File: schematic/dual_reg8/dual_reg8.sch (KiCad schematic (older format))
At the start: 52 parts

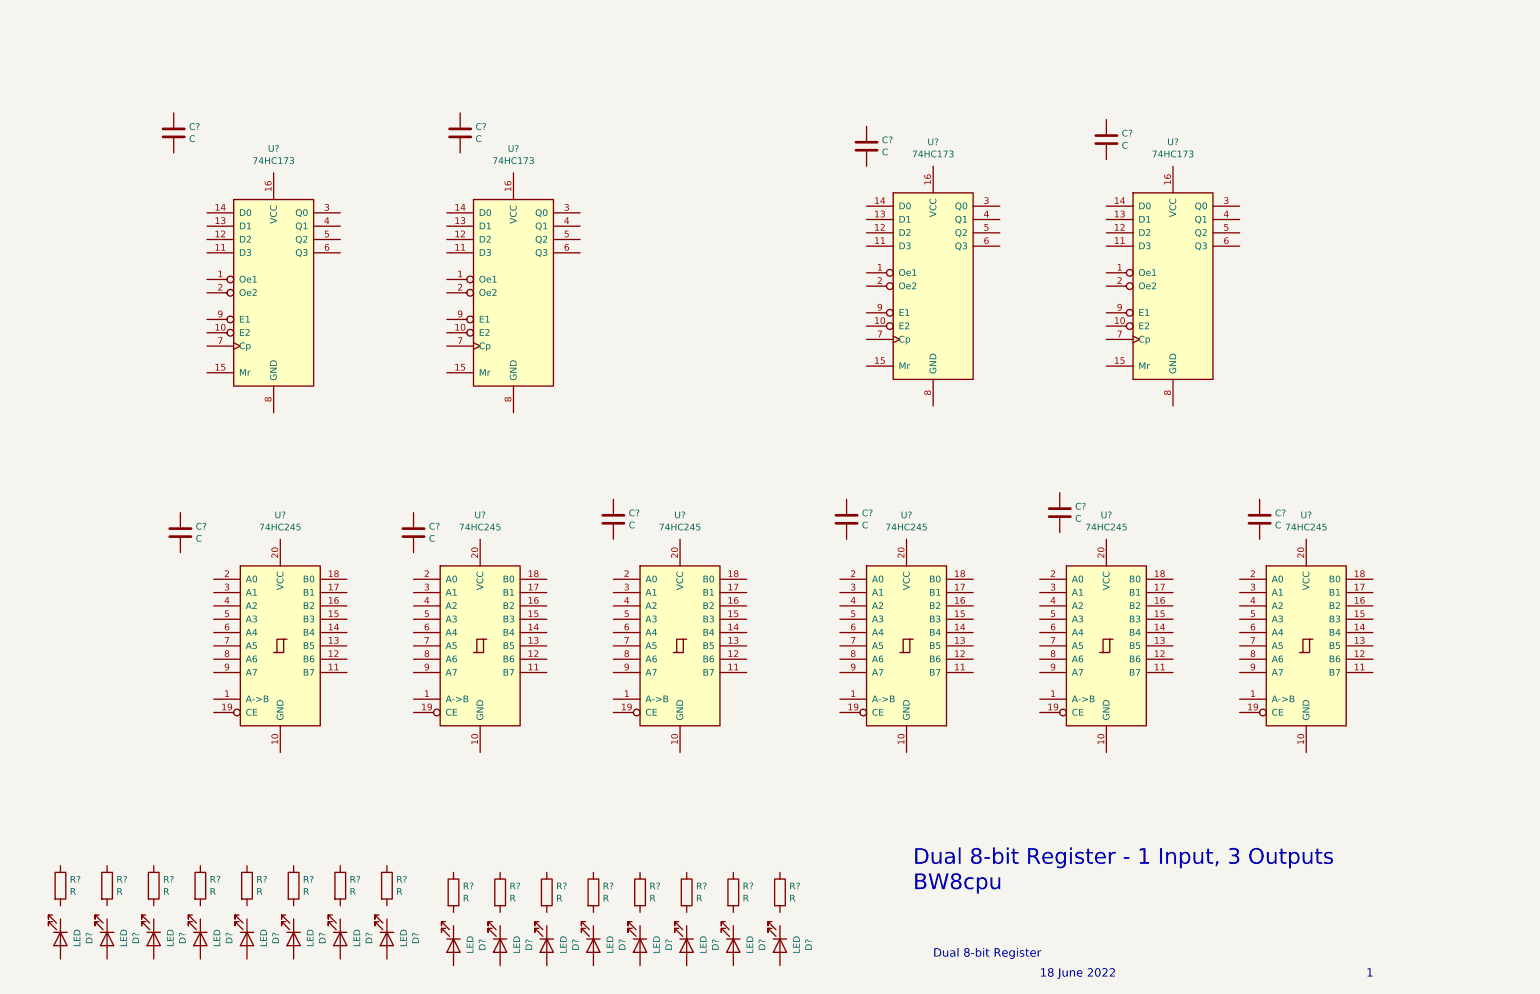
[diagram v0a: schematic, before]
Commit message: switching branches, cleaning tree
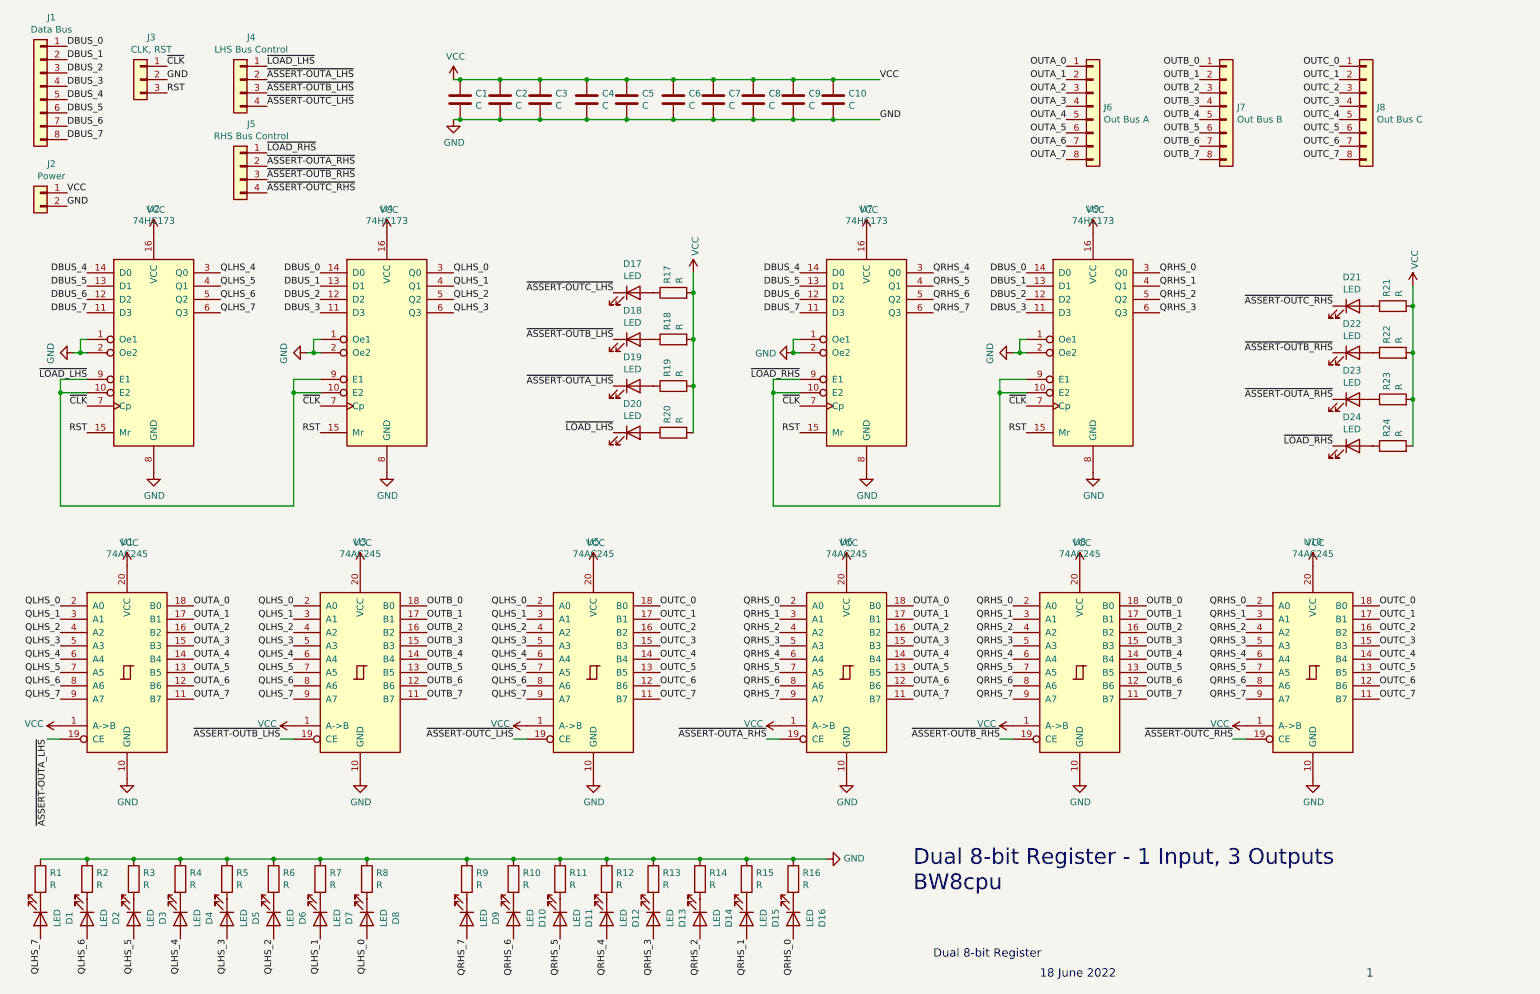
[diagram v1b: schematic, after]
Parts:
- removed C? (x9): C, symbol Device:C
- removed D? (x15): LED, symbol Device:LED
- removed R? (x15): R, symbol Device:R
- removed U? (x2): 74HC173, symbol 74xx:74LS173
- removed U? (x3): 74HC245, symbol 74xx:74HC245
- added C10, C2, C3, C4, C5, C6, C7, C8, C9: C, Capacitor_THT:C_Disc_D3.0mm_W1.6mm_P2.50mm, symbol Device:C
- added D10, D11, D12, D13, D14, D15, D16, D17, D18, D19, D2, D20, D21, D22, D23, D24, D3, D4, D5, D6, D7, D8, D9: LED, LED_THT:LED_D2.0mm_W4.8mm_H2.5mm_FlatTop, symbol Device:LED
- added J1: Data Bus, Connector_PinSocket_2.54mm:PinSocket_1x08_P2.54mm_Vertical, symbol Connector_Generic:Conn_01x08
- added J2: Power, Connector_PinSocket_2.54mm:PinSocket_1x02_P2.54mm_Vertical, symbol Connector_Generic:Conn_01x02
- added J3: CLK, RST, Connector_PinSocket_2.54mm:PinSocket_1x03_P2.54mm_Vertical, symbol Connector_Generic:Conn_01x03
- added J4: LHS Bus Control, Connector_PinSocket_2.54mm:PinSocket_1x04_P2.54mm_Vertical, symbol Connector_Generic:Conn_01x04
- added J5: RHS Bus Control, Connector_PinSocket_2.54mm:PinSocket_1x04_P2.54mm_Vertical, symbol Connector_Generic:Conn_01x04
- added J6: Out Bus A, Connector_PinSocket_2.54mm:PinSocket_1x08_P2.54mm_Vertical, symbol Connector_Generic:Conn_01x08
- added J7: Out Bus B, Connector_PinSocket_2.54mm:PinSocket_1x08_P2.54mm_Vertical, symbol Connector_Generic:Conn_01x08
- added J8: Out Bus C, Connector_PinSocket_2.54mm:PinSocket_1x08_P2.54mm_Vertical, symbol Connector_Generic:Conn_01x08
- added R10, R11, R12, R13, R14, R15, R16, R17, R18, R19, R2, R20, R21, R22, R23, R24, R3, R4, R5, R6, R7, R8, R9: R, Resistor_THT:R_Axial_DIN0204_L3.6mm_D1.6mm_P5.08mm_Horizontal, symbol Device:R
- added U10, U6, U8: 74AC245, Package_DIP:DIP-20_W7.62mm, symbol 74xx:74HC245
- added U7, U9: 74HC173, Package_DIP:DIP-16_W7.62mm, symbol 74xx:74LS173
- C1: renamed from C?; footprint (none) -> Capacitor_THT:C_Disc_D3.0mm_W1.6mm_P2.50mm
- D1: renamed from D?; footprint (none) -> LED_THT:LED_D2.0mm_W4.8mm_H2.5mm_FlatTop
- R1: renamed from R?; footprint (none) -> Resistor_THT:R_Axial_DIN0204_L3.6mm_D1.6mm_P5.08mm_Horizontal
- U1, U3, U5: renamed from U?; value 74HC245 -> 74AC245; footprint (none) -> Package_DIP:DIP-20_W7.62mm
- U2, U4: renamed from U?; footprint (none) -> Package_DIP:DIP-16_W7.62mm
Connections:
- net GND: now reaches U2.1 (Oe1)
- net GND: now also C1.2, R1.1, U1.10 (GND), U2.2 (Oe2), U2.8 (GND), U3.10 (GND), U4.1 (Oe1), U4.2 (Oe2), U4.8 (GND), U5.10 (GND), C10.2, C2.2, C3.2, C4.2, C5.2, C6.2, C7.2, C8.2, C9.2, J2.2 (Pin_2), J3.2 (Pin_2), R10.1, R11.1, R12.1, R13.1, R14.1, R15.1, R16.1, R2.1, R3.1, R4.1, R5.1, R6.1, R7.1, R8.1, R9.1, U10.10 (GND), U6.10 (GND), U7.1 (Oe1), U7.2 (Oe2), U7.8 (GND), U8.10 (GND), U9.1 (Oe1), U9.2 (Oe2), U9.8 (GND)
- net ~LOAD_LHS: now reaches U2.10 (E2)
- net ~LOAD_LHS: now also U2.9 (E1), U4.10 (E2), U4.9 (E1), D20.1 (K), J4.1 (Pin_1)
- net DBUS_7: now reaches U2.11 (D3)
- net DBUS_7: now also J1.8 (Pin_8), U7.11 (D3)
- net DBUS_6: now reaches U2.12 (D2)
- net DBUS_6: now also J1.7 (Pin_7), U7.12 (D2)
- net DBUS_5: now reaches U2.13 (D1)
- net DBUS_5: now also J1.6 (Pin_6), U7.13 (D1)
- net DBUS_4: now reaches U2.14 (D0)
- net DBUS_4: now also J1.5 (Pin_5), U7.14 (D0)
- net RST: now reaches U2.15 (Mr)
- net RST: now also U4.15 (Mr), J3.3 (Pin_3), U7.15 (Mr), U9.15 (Mr)
- net VCC: now reaches U2.16 (VCC)
- net VCC: now also C1.1, U1.1 (A->B), U1.20 (VCC), U3.1 (A->B), U3.20 (VCC), U4.16 (VCC), U5.1 (A->B), U5.20 (VCC), C10.1, C2.1, C3.1, C4.1, C5.1, C6.1, C7.1, C8.1, C9.1, J2.1 (Pin_1), R17.2, R18.2, R19.2, R20.2, R21.2, R22.2, R23.2, R24.2, U10.1 (A->B), U10.20 (VCC), U6.1 (A->B), U6.20 (VCC), U7.16 (VCC), U8.1 (A->B), U8.20 (VCC), U9.16 (VCC)
- net QLHS_4: now reaches U2.3 (Q0)
- net QLHS_4: now also U1.6 (A4), U3.6 (A4), U5.6 (A4), D4.2 (A)
- net QLHS_5: now reaches U2.4 (Q1)
- net QLHS_5: now also U1.7 (A5), U3.7 (A5), U5.7 (A5), D3.2 (A)
- net QLHS_6: now reaches U2.5 (Q2)
- net QLHS_6: now also U1.8 (A6), U3.8 (A6), U5.8 (A6), D2.2 (A)
- net QLHS_7: now reaches U2.6 (Q3)
- net QLHS_7: now also D1.2 (A), U1.9 (A7), U3.9 (A7), U5.9 (A7)
- net ~CLK: now reaches U2.7 (Cp)
- net ~CLK: now also U4.7 (Cp), J3.1 (Pin_1), U7.7 (Cp), U9.7 (Cp)
- net DBUS_3: now reaches U4.11 (D3)
- net DBUS_3: now also J1.4 (Pin_4), U9.11 (D3)
- net DBUS_2: now reaches U4.12 (D2)
- net DBUS_2: now also J1.3 (Pin_3), U9.12 (D2)
- net DBUS_1: now reaches U4.13 (D1)
- net DBUS_1: now also J1.2 (Pin_2), U9.13 (D1)
- net DBUS_0: now reaches U4.14 (D0)
- net DBUS_0: now also J1.1 (Pin_1), U9.14 (D0)
- net QLHS_0: now reaches U4.3 (Q0)
- net QLHS_0: now also U1.2 (A0), U3.2 (A0), U5.2 (A0), D8.2 (A)
- net QLHS_1: now reaches U4.4 (Q1)
- net QLHS_1: now also U1.3 (A1), U3.3 (A1), U5.3 (A1), D7.2 (A)
- net QLHS_2: now reaches U4.5 (Q2)
- net QLHS_2: now also U1.4 (A2), U3.4 (A2), U5.4 (A2), D6.2 (A)
- net QLHS_3: now reaches U4.6 (Q3)
- net QLHS_3: now also U1.5 (A3), U3.5 (A3), U5.5 (A3), D5.2 (A)
- net OUTA_7: now reaches U1.11 (B7)
- net OUTA_7: now also J6.8 (Pin_8), U6.11 (B7)
- net OUTA_6: now reaches U1.12 (B6)
- net OUTA_6: now also J6.7 (Pin_7), U6.12 (B6)
- net OUTA_5: now reaches U1.13 (B5)
- net OUTA_5: now also J6.6 (Pin_6), U6.13 (B5)
- net OUTA_4: now reaches U1.14 (B4)
- net OUTA_4: now also J6.5 (Pin_5), U6.14 (B4)
- net OUTA_3: now reaches U1.15 (B3)
- net OUTA_3: now also J6.4 (Pin_4), U6.15 (B3)
- net OUTA_2: now reaches U1.16 (B2)
- net OUTA_2: now also J6.3 (Pin_3), U6.16 (B2)
- net OUTA_1: now reaches U1.17 (B1)
- net OUTA_1: now also J6.2 (Pin_2), U6.17 (B1)
- net OUTA_0: now reaches U1.18 (B0)
- net OUTA_0: now also J6.1 (Pin_1), U6.18 (B0)
- net ~ASSERT-OUTA_LHS: now reaches U1.19 (CE)
- net ~ASSERT-OUTA_LHS: now also D19.1 (K), J4.2 (Pin_2)
- net OUTB_7: now reaches U3.11 (B7)
- net OUTB_7: now also J7.8 (Pin_8), U8.11 (B7)
- net OUTB_6: now reaches U3.12 (B6)
- net OUTB_6: now also J7.7 (Pin_7), U8.12 (B6)
- net OUTB_5: now reaches U3.13 (B5)
- net OUTB_5: now also J7.6 (Pin_6), U8.13 (B5)
- net OUTB_4: now reaches U3.14 (B4)
- net OUTB_4: now also J7.5 (Pin_5), U8.14 (B4)
- net OUTB_3: now reaches U3.15 (B3)
- net OUTB_3: now also J7.4 (Pin_4), U8.15 (B3)
- net OUTB_2: now reaches U3.16 (B2)
- net OUTB_2: now also J7.3 (Pin_3), U8.16 (B2)
- net OUTB_1: now reaches U3.17 (B1)
- net OUTB_1: now also J7.2 (Pin_2), U8.17 (B1)
- net OUTB_0: now reaches U3.18 (B0)
- net OUTB_0: now also J7.1 (Pin_1), U8.18 (B0)
- net ~ASSERT-OUTB_LHS: now reaches U3.19 (CE)
- net ~ASSERT-OUTB_LHS: now also D18.1 (K), J4.3 (Pin_3)
- net OUTC_7: now reaches U5.11 (B7)
- net OUTC_7: now also J8.8 (Pin_8), U10.11 (B7)
- net OUTC_6: now reaches U5.12 (B6)
- net OUTC_6: now also J8.7 (Pin_7), U10.12 (B6)
- net OUTC_5: now reaches U5.13 (B5)
- net OUTC_5: now also J8.6 (Pin_6), U10.13 (B5)
- net OUTC_4: now reaches U5.14 (B4)
- net OUTC_4: now also J8.5 (Pin_5), U10.14 (B4)
- net OUTC_3: now reaches U5.15 (B3)
- net OUTC_3: now also J8.4 (Pin_4), U10.15 (B3)
- net OUTC_2: now reaches U5.16 (B2)
- net OUTC_2: now also J8.3 (Pin_3), U10.16 (B2)
- net OUTC_1: now reaches U5.17 (B1)
- net OUTC_1: now also J8.2 (Pin_2), U10.17 (B1)
- net OUTC_0: now reaches U5.18 (B0)
- net OUTC_0: now also J8.1 (Pin_1), U10.18 (B0)
- net ~ASSERT-OUTC_LHS: now reaches U5.19 (CE)
- net ~ASSERT-OUTC_LHS: now also D17.1 (K), J4.4 (Pin_4)
- net at D1.1 (K): now also R1.2
- new net: D2.1 (K), R2.2
- new net: D3.1 (K), R3.2
- new net: D4.1 (K), R4.2
- new net: D5.1 (K), R5.2
- new net: D6.1 (K), R6.2
- new net: D7.1 (K), R7.2
- new net: D8.1 (K), R8.2
- new net: D9.1 (K), R9.2
- new net: D10.1 (K), R10.2
- new net: D11.1 (K), R11.2
- new net: D12.1 (K), R12.2
- new net: D13.1 (K), R13.2
- new net: D14.1 (K), R14.2
- new net: D15.1 (K), R15.2
- new net: D16.1 (K), R16.2
- new net: D20.2 (A), R20.1
- new net: D19.2 (A), R19.1
- new net: D18.2 (A), R18.1
- new net: D17.2 (A), R17.1
- new net: D24.2 (A), R24.1
- new net: D23.2 (A), R23.1
- new net: D22.2 (A), R22.1
- new net: D21.2 (A), R21.1
- new net QRHS_0: D16.2 (A), U10.2 (A0), U6.2 (A0), U8.2 (A0), U9.3 (Q0)
- new net QRHS_1: D15.2 (A), U10.3 (A1), U6.3 (A1), U8.3 (A1), U9.4 (Q1)
- new net QRHS_2: D14.2 (A), U10.4 (A2), U6.4 (A2), U8.4 (A2), U9.5 (Q2)
- new net QRHS_3: D13.2 (A), U10.5 (A3), U6.5 (A3), U8.5 (A3), U9.6 (Q3)
- new net QRHS_4: D12.2 (A), U10.6 (A4), U6.6 (A4), U7.3 (Q0), U8.6 (A4)
- new net QRHS_5: D11.2 (A), U10.7 (A5), U6.7 (A5), U7.4 (Q1), U8.7 (A5)
- new net QRHS_6: D10.2 (A), U10.8 (A6), U6.8 (A6), U7.5 (Q2), U8.8 (A6)
- new net QRHS_7: D9.2 (A), U10.9 (A7), U6.9 (A7), U7.6 (Q3), U8.9 (A7)
- new net ~ASSERT-OUTA_RHS: D23.1 (K), J5.2 (Pin_2), U6.19 (CE)
- new net ~ASSERT-OUTB_RHS: D22.1 (K), J5.3 (Pin_3), U8.19 (CE)
- new net ~ASSERT-OUTC_RHS: D21.1 (K), J5.4 (Pin_4), U10.19 (CE)
- new net ~LOAD_RHS: D24.1 (K), J5.1 (Pin_1), U7.10 (E2), U7.9 (E1), U9.10 (E2), U9.9 (E1)
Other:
- moved on the sheet: C1, D1, R1, U1, U2, U3, U4, U5
